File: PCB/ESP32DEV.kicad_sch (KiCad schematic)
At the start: 32 parts, among them J1 USB_C_Receptacle_USB2.0_16P, J2 Conn_01x18_Pin, J3 Conn_01x18_Pin, J5 Conn_01x04_Pin, J6 Conn_01x02_Pin, Q1 AO3401A, SW1 SW_Push, SW2 SW_Push, U2 AP63203WU, U5 ESP32-S3-WROOM-1

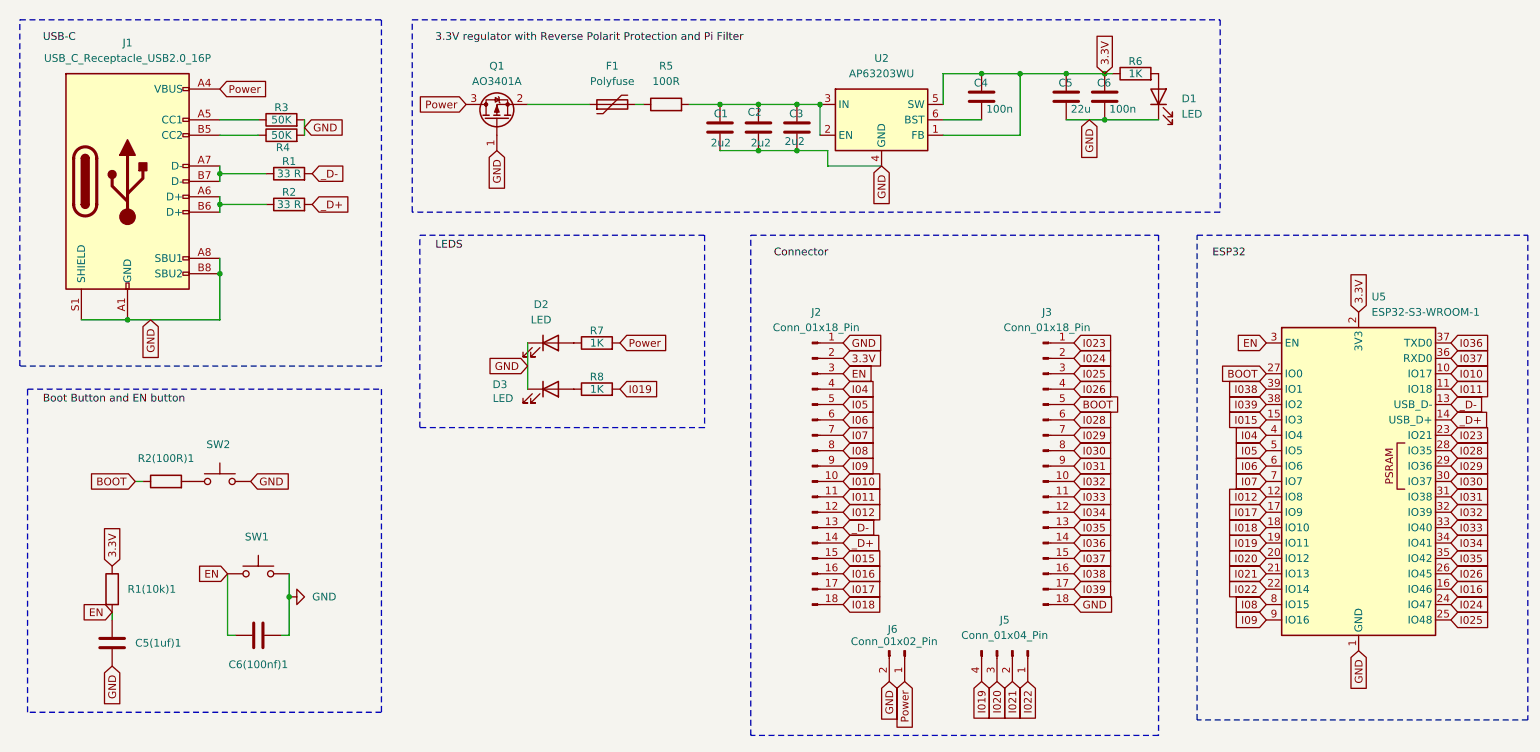
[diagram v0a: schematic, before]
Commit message: Add files via upload
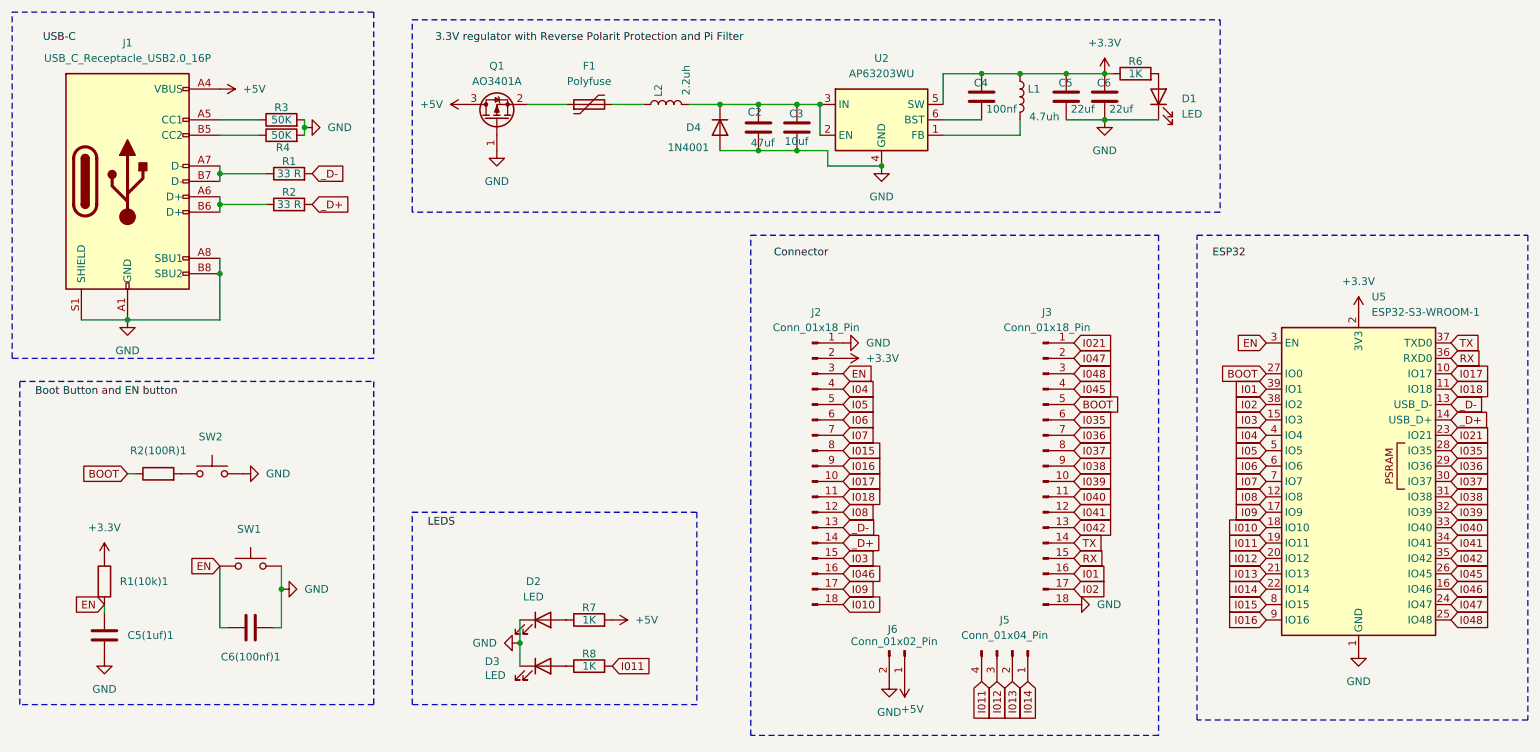
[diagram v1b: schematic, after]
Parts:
- removed C1: 2u2, Capacitor_SMD:C_0201_0603Metric, symbol Device:C
- removed R5: 100R, Resistor_SMD:R_0603_1608Metric, symbol Device:R
- added D4: 1N4001, Diode_THT:D_DO-41_SOD81_P2.54mm_Vertical_AnodeUp, symbol Diode:1N4001
- added L1: 4.7uh, Inductor_SMD:L_0603_1608Metric, symbol Device:L
- added L2: 2.2uh, Inductor_SMD:L_0603_1608Metric, symbol Device:L
- C2: value 2u2 -> 47uf
- C3: value 2u2 -> 10uf
- C4: value 100n -> 100nf
- C5: value 22u -> 22uf
- C6: value 100n -> 22uf
- R1, R2, R3, R4: footprint Resistor_SMD:R_0201_0603Metric_Pad0.64x0.40mm_HandSolder -> Resistor_SMD:R_0603_1608Metric
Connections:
- net I019 is gone; now on net I011: J5.4 (Pin_4), R8.2, U5.19 (IO11)
- net I020 is gone; now on net I012: J5.3 (Pin_3), U5.20 (IO12)
- net I023 is gone; now on net I021: J3.1 (Pin_1), U5.23 (IO21)
- net I028 is gone; now on net I035: J3.6 (Pin_6), U5.28 (IO35)
- net I029 is gone; now on net I036: J3.7 (Pin_7), U5.29 (IO36)
- net I030 is gone; now on net I037: J3.8 (Pin_8), U5.30 (IO37)
- net I031 is gone; now on net I038: J3.9 (Pin_9), U5.31 (IO38)
- net I032 is gone; now on net I039: J3.10 (Pin_10), U5.32 (IO39)
- net GND: now also D4.2 (A)
- net I010: now also J2.18 (Pin_18), U5.18 (IO10); no longer J2.10 (Pin_10), U5.10 (IO17)
- net I011: no longer J2.11 (Pin_11), U5.11 (IO18)
- net I012: no longer J2.12 (Pin_12), U5.12 (IO8)
- net I015: now also J2.8 (Pin_8), U5.8 (IO15); no longer J2.15 (Pin_15), U5.15 (IO3)
- net I016: now also J2.9 (Pin_9), U5.9 (IO16); no longer J2.16 (Pin_16), U5.16 (IO46)
- net I017: now also J2.10 (Pin_10), U5.10 (IO17); no longer J2.17 (Pin_17), U5.17 (IO9)
- net I018: now also J2.11 (Pin_11), U5.11 (IO18); no longer J2.18 (Pin_18), U5.18 (IO10)
- net I021: no longer J5.2 (Pin_2), U5.21 (IO13)
- net I035: no longer J3.13 (Pin_13), U5.35 (IO42)
- net I036: no longer J3.14 (Pin_14), U5.37 (TXD0)
- net I037: no longer J3.15 (Pin_15), U5.36 (RXD0)
- net I038: no longer J3.16 (Pin_16), U5.39 (IO1)
- net I039: no longer J3.17 (Pin_17), U5.38 (IO2)
- net I08: now also J2.12 (Pin_12), U5.12 (IO8); no longer J2.8 (Pin_8), U5.8 (IO15)
- net I09: now also J2.17 (Pin_17), U5.17 (IO9); no longer J2.9 (Pin_9), U5.9 (IO16)
- net at C2.1, C3.1, U2.2 (EN)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: now also D4.1 (K), L2.2
- net at F1.2: now also L2.1
- net 3.3V renamed +3.3V
- net +3.3V: now also L1.1; no longer U2.1 (FB)
- net I022 renamed I014
- net I024 renamed I047
- net I025 renamed I048
- net I026 renamed I045
- net I033 renamed I040
- net I034 renamed I041
- net Power renamed +5V
- new net: L1.2, U2.1 (FB)
- new net I01: J3.16 (Pin_16), U5.39 (IO1)
- new net I013: J5.2 (Pin_2), U5.21 (IO13)
- new net I02: J3.17 (Pin_17), U5.38 (IO2)
- new net I03: J2.15 (Pin_15), U5.15 (IO3)
- new net I042: J3.13 (Pin_13), U5.35 (IO42)
- new net I046: J2.16 (Pin_16), U5.16 (IO46)
- new net RX: J3.15 (Pin_15), U5.36 (RXD0)
- new net TX: J3.14 (Pin_14), U5.37 (TXD0)
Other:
- moved on the sheet: C5(1uf)1, C6(100nf)1, D2, D3, F1, R1(10k)1, R2(100R)1, R7, R8, SW1, SW2
